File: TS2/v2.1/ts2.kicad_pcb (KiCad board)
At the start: 2 copper layers, 134.6 x 208.3 mm, 110 parts, among them P1 FTDI (TERMINAL), P2 FTDI (HOST), P3 +5V POWER, SW1 RESET, SW2 SINGLE STEP/RUN, SW3 STEP, SW4 ABORT, SW5 POWER, U1 555, U10 74LS32, U11 HM6264, U12 28C64, U13 HM6264, U14 28C64, U15 HM6264, U16 28C64, U17 HM6264, U18 28C64, U19 74LS20, U2 8 MHz, U20 74LS74, U21 74LS161, U22 74LS161, U23 74LS74, U24 74LS260, U25 74LS260, U26 74LS138, U27 74LS138, U28 74LS148, U29 6850, U3 74LS00, U30 6850, U31 74HC4060, U32 74LS138, U33 74LS138, U34 74LS00, U35 74LS74, U36 74LS27, U37 74LS00, U4 74LS06, U5 74LS04, U6 68000, U7 74LS08, U8 74LS32, U9 74LS32, Y1 2.4576MHz

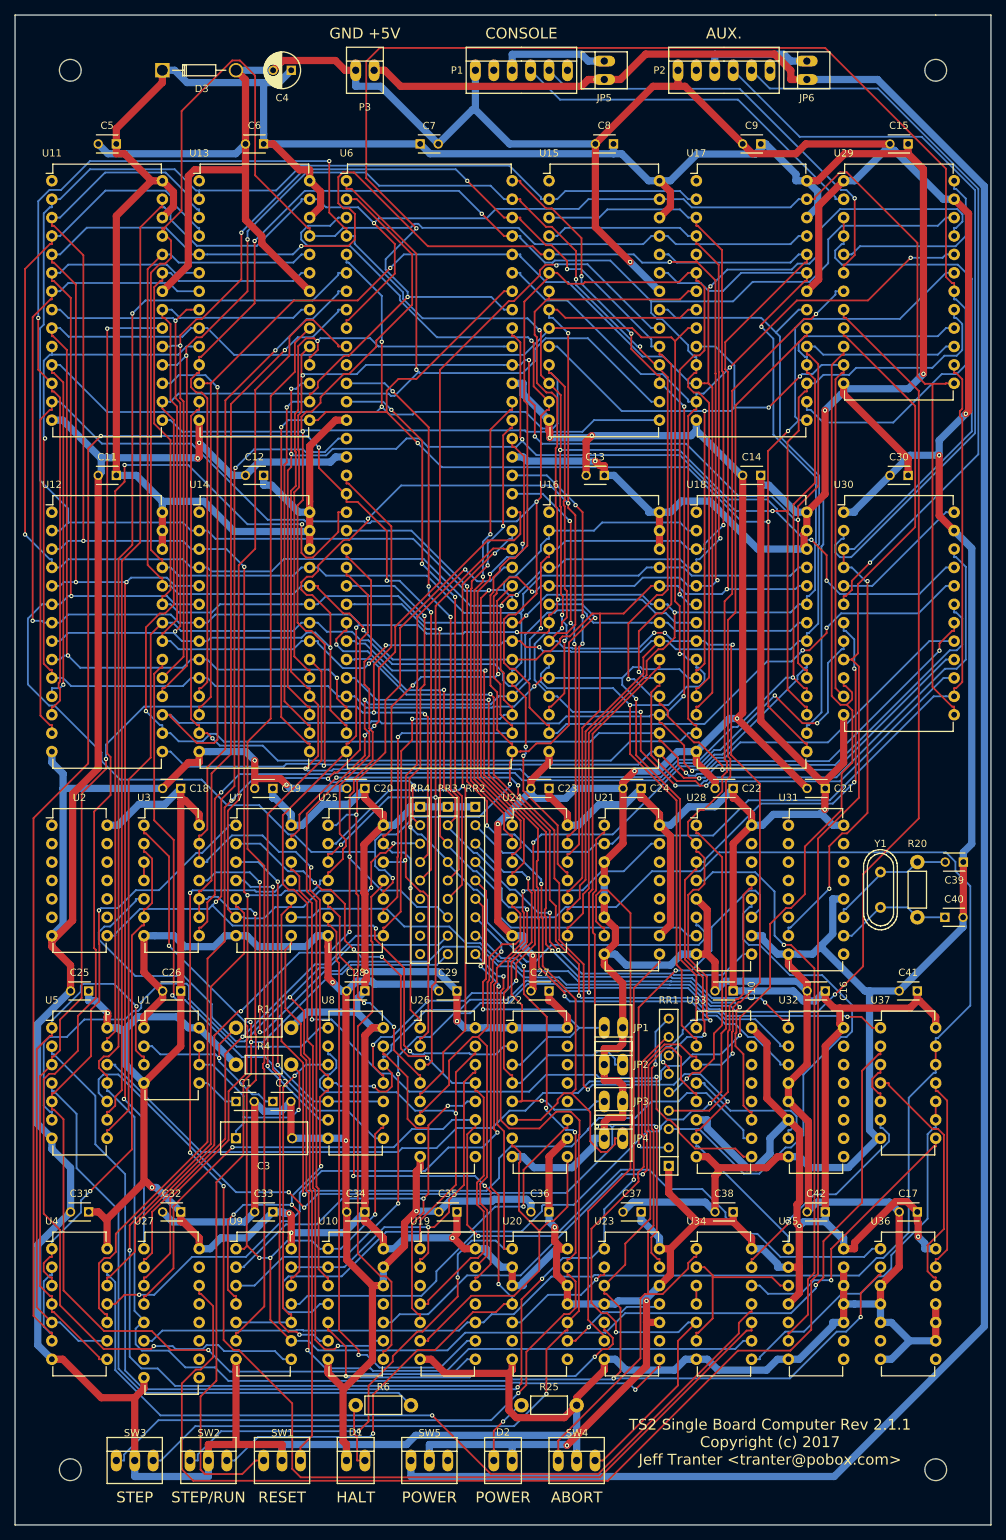
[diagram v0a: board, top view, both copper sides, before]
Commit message: add updated gerber & drill files
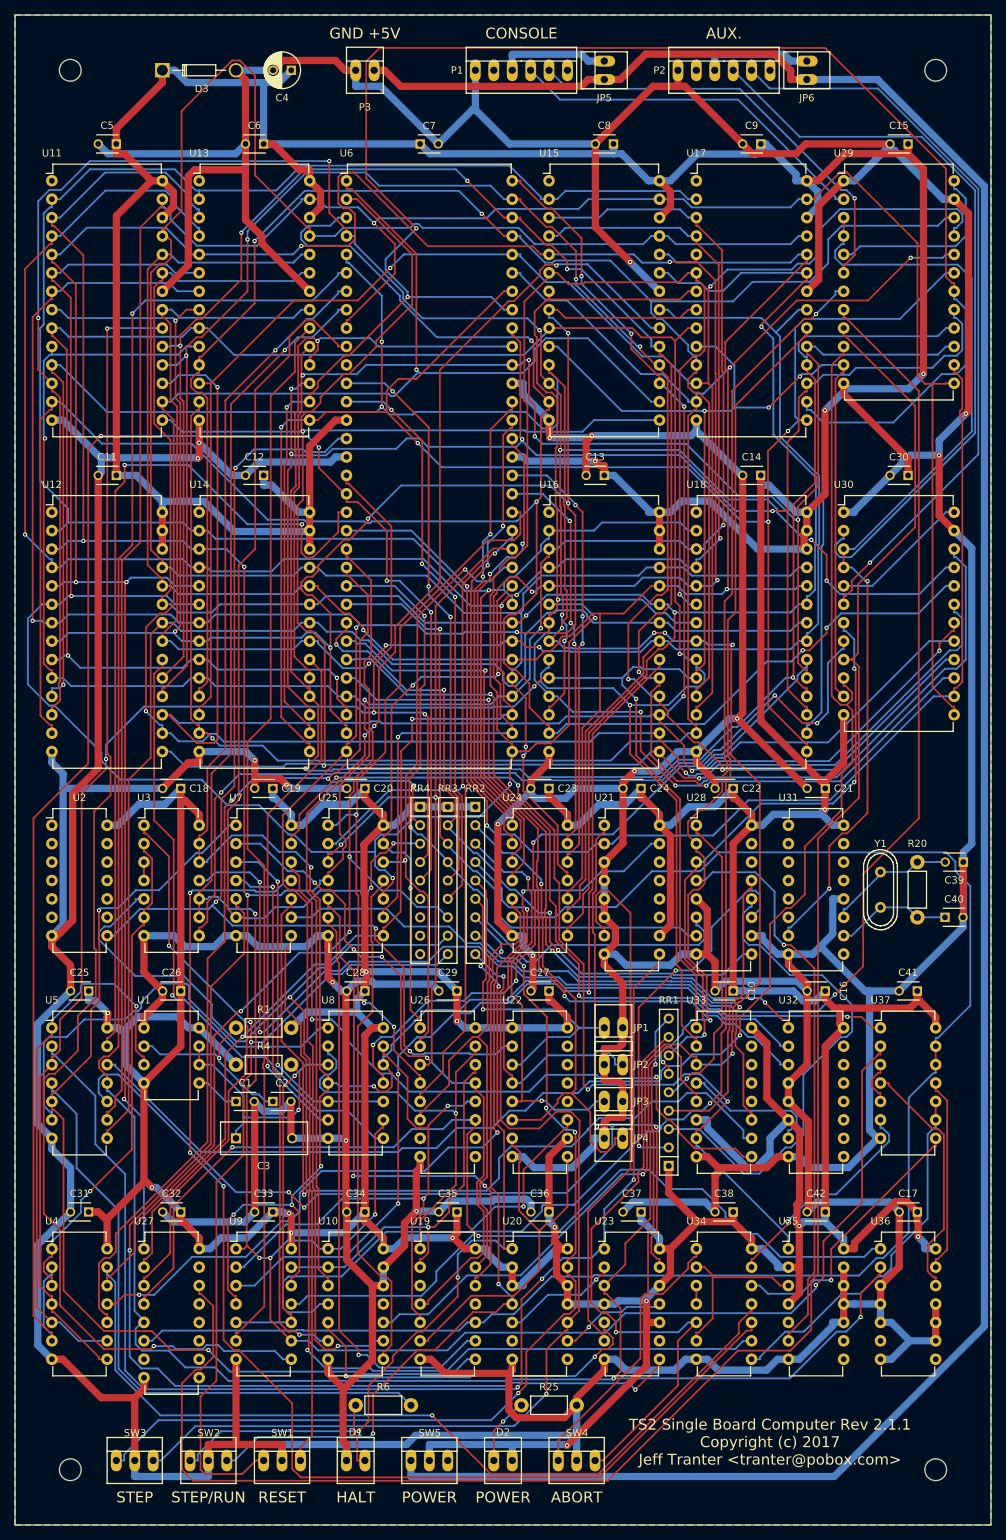
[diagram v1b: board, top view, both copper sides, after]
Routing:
- added copper zone on B.Cu, net GND
- added copper zone on F.Cu, net GND
